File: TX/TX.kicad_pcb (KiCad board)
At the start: 2 copper layers, 95.2 x 73.7 mm, 41 parts, among them J2 ANT, Q1 BS170, Q4 BS170, Q5 BS170, Q6 BS170, SW1 Start/Stop, SW2 ON, SW3 EXT, T1 2 x 10 @ FT37-43, T2 3 x 8T @ FT37-43, U1 ATtiny45-20PU, U2 L78L05, Y1 14.31818MHz

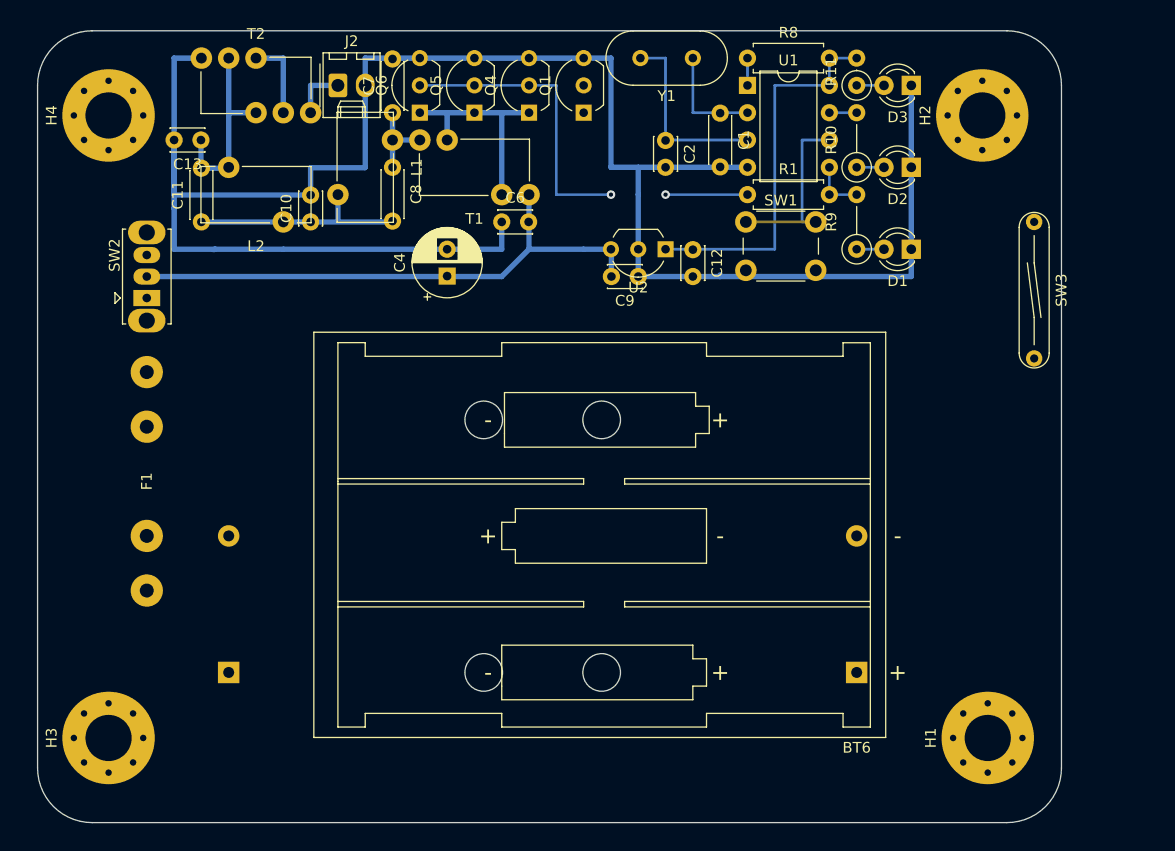
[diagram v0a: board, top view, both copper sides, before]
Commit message: Tiny release.
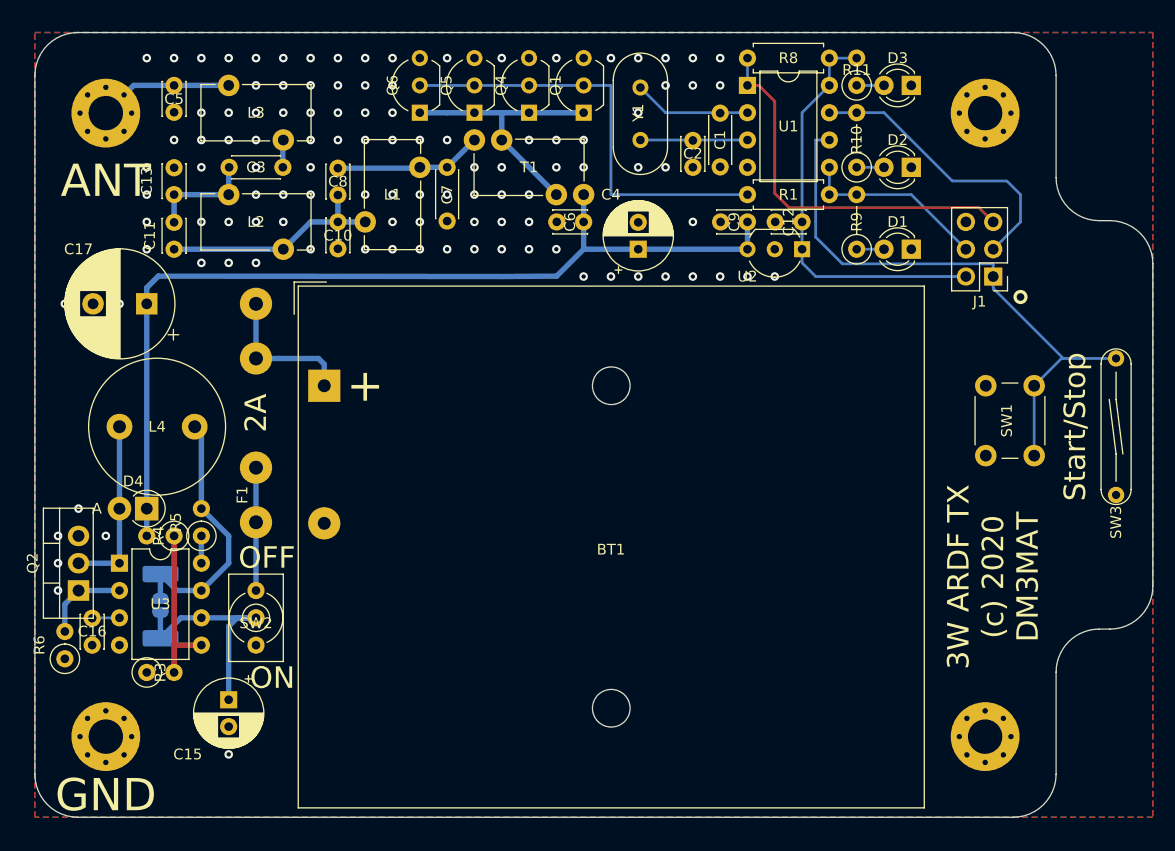
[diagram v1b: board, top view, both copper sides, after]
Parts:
- removed BT6: 3.6V, Battery:BatteryHolder_Keystone_2479_3xAAA
- removed J2: ANT, Connector_Molex:Molex_KK-254_AE-6410-02A_1x02_P2.54mm_Vertical
- removed T2: 3 x 8T @ FT37-43, DM3MAT:Transformer_1P_2S_Toroid_Vertical_D10.5mm_Amidon-T37
- added C15: 220u, Capacitor_THT:CP_Radial_D6.3mm_P2.50mm, F.Cu at (113.0, 130.8)
- added C16: 470p, Capacitor_THT:C_Disc_D3.0mm_W2.0mm_P2.50mm, F.Cu at (100.3, 123.2)
- added C17: 470u, Capacitor_THT:CP_Radial_D10.0mm_P5.00mm, F.Cu at (105.4, 94.0)
- added C3: 220n, Capacitor_THT:C_Disc_D4.3mm_W1.9mm_P5.00mm, F.Cu at (113.1, 81.3)
- added C5: 47p, Capacitor_THT:C_Disc_D3.0mm_W2.0mm_P2.50mm, F.Cu at (108.0, 73.7)
- added D4: 1N5819, Diode_THT:D_DO-41_SOD81_P2.54mm_Vertical_AnodeUp, F.Cu at (105.4, 113.0)
- added J1: AVR-ISP-6, Connector_PinHeader_2.54mm:PinHeader_2x03_P2.54mm_Vertical, F.Cu at (184.2, 91.4)
- added JP1: SolderJumper_2_Open, Jumper:SolderJumper-2_P1.3mm_Open_RoundedPad1.0x1.5mm, B.Cu at (106.7, 122.0)
- added L3: 42u, DM3MAT:L_Toroid_Vertical_L10.0mm_W5.0mm_P5.08mm_Diagonal, F.Cu at (115.6, 76.2)
- added L4: 20uH, Inductor_THT:L_Radial_D12.5mm_P7.00mm_Fastron_09HCP, F.Cu at (109.9, 105.4)
- added Q2: TIP41, Package_TO_SOT_THT:TO-220-3_Vertical, F.Cu at (99.1, 120.7)
- added R2: 0.2, Resistor_SMD:R_2512_6332Metric_Pad1.52x3.35mm_HandSolder, B.Cu at (106.7, 122.1)
- added R3: 1k, Resistor_THT:R_Axial_DIN0207_L6.3mm_D2.5mm_P2.54mm_Vertical, F.Cu at (105.4, 128.3)
- added R4: 6.2k, Resistor_THT:R_Axial_DIN0207_L6.3mm_D2.5mm_P2.54mm_Vertical, F.Cu at (108.0, 115.6)
- added R5: 180, Resistor_THT:R_Axial_DIN0207_L6.3mm_D2.5mm_P2.54mm_Vertical, F.Cu at (110.5, 115.6)
- added R6: 22, Resistor_THT:R_Axial_DIN0207_L6.3mm_D2.5mm_P2.54mm_Vertical, F.Cu at (97.8, 127.0)
- added U3: MC34063AP, Package_DIP:DIP-8_W7.62mm, F.Cu at (102.9, 118.1)
- BT1: footprint Battery:BatteryHolder_Keystone_2479_3xAAA -> Battery:BatteryHolder_TruPower_BH-331P_3xAA; moved to F.Cu
- C11, C8: footprint Capacitor_THT:C_Disc_D4.3mm_W1.9mm_P5.00mm -> Capacitor_THT:C_Disc_D3.0mm_W2.0mm_P2.50mm
- F1: value 1A Flink -> 2A Träge
- H1, H2, H3: footprint MountingHole:MountingHole_4.3mm_M4_Pad_Via -> MountingHole:MountingHole_3.2mm_M3_Pad_Via
- H4: value GND -> ANT; footprint MountingHole:MountingHole_4.3mm_M4_Pad_Via -> MountingHole:MountingHole_3.2mm_M3_Pad_Via
- R1: value 2.2k -> 100
- SW2: footprint Button_Switch_THT:SW_Slide_1P2T_CK_OS102011MS2Q -> DM3MAT:SW_Lever_RND-210-004371
- moved SW2 31.4 mm to (115.6, 123.2), turned to 0 degrees
- moved SW1 30.8 mm to (188.0, 101.6), turned to 270 degrees
- moved BT1 28.1 mm to (121.9, 101.6)
- moved C4 18.0 mm to (151.1, 88.9)
- moved SW3 14.8 mm to (195.6, 105.4)
- moved U2 12.7 mm to (166.4, 88.9)
- moved C12 10.5 mm to (166.4, 86.4), turned to 180 degrees
- moved C9 9.19 mm to (158.8, 86.4), turned to 0 degrees
- moved C7 7.18 mm to (133.3, 81.3), turned to 270 degrees
- moved F1 6.84 mm to (109.2, 104.1), turned to 90 degrees
- moved C13 5.66 mm to (108.0, 83.8), turned to 90 degrees
- moved Y1 5.60 mm to (151.3, 73.9), turned to 270 degrees
- moved C6 5.12 mm to (143.6, 86.4)
- moved C8 5.08 mm to (123.2, 81.4)
- moved T1 5.08 mm to (141.0, 83.8)
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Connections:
- net ACT renamed LED
- F1 pad 2: Net-(BT6-Pad1) -> Net-(BT1-Pad1)
- H4 pad 1: GND -> Net-(C5-Pad1)
- SW2 pad 2: VCC -> Net-(C15-Pad1)
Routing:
- net GND: track 189.5 -> 0.00 mm, vias 0 -> 115
- net SS: track 17.9 -> 54.3 mm
- net VCC: track 51.9 -> 88.1 mm
- net RST: track 2.54 -> 35.7 mm
- net LED: track 2.54 -> 27.1 mm
- net Net-(JP1-Pad2): track 0.00 -> 24.3 mm
- net Net-(C15-Pad1): track 0.00 -> 21.8 mm
- net Net-(D4-Pad2): track 0.00 -> 16.5 mm
- net Net-(R3-Pad2): track 0.00 -> 15.2 mm
- net Net-(BT1-Pad1): track 0.00 -> 13.7 mm
- net Net-(C5-Pad1): track 0.00 -> 12.5 mm
- net KEY: track 5.08 -> 17.3 mm
- net Net-(F1-Pad1): track 0.00 -> 11.4 mm
- net Net-(Q2-Pad1): track 0.00 -> 8.15 mm
- net Xo: track 17.6 -> 9.96 mm
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- added copper zone on B.Cu, net GND
- added copper zone on F.Cu, net GND
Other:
- board size 95.2 x 73.7 mm -> 104 x 73 mm
- board text added: "2A"
- board text added: "3W ARDF TX (c) 2020 DM3MAT"
- board text added: "ANT"
- board text added: "GND"
- board text added: "OFF"
- board text added: "ON"
- board text added: "Start/Stop"
